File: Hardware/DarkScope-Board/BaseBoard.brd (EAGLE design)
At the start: 101.9 x 80 mm, 85 parts, among them IC1 7805DT, IC2 REG1117, IC3 7905, J1 DCJ0202, Q1 8MHz, T2 9014, U1 STM32F103CBT6, X1 TSW-102-07-G-S, X2 TSW-102-07-G-S, X3 MINI-USB-32005-301, X4 2540-5

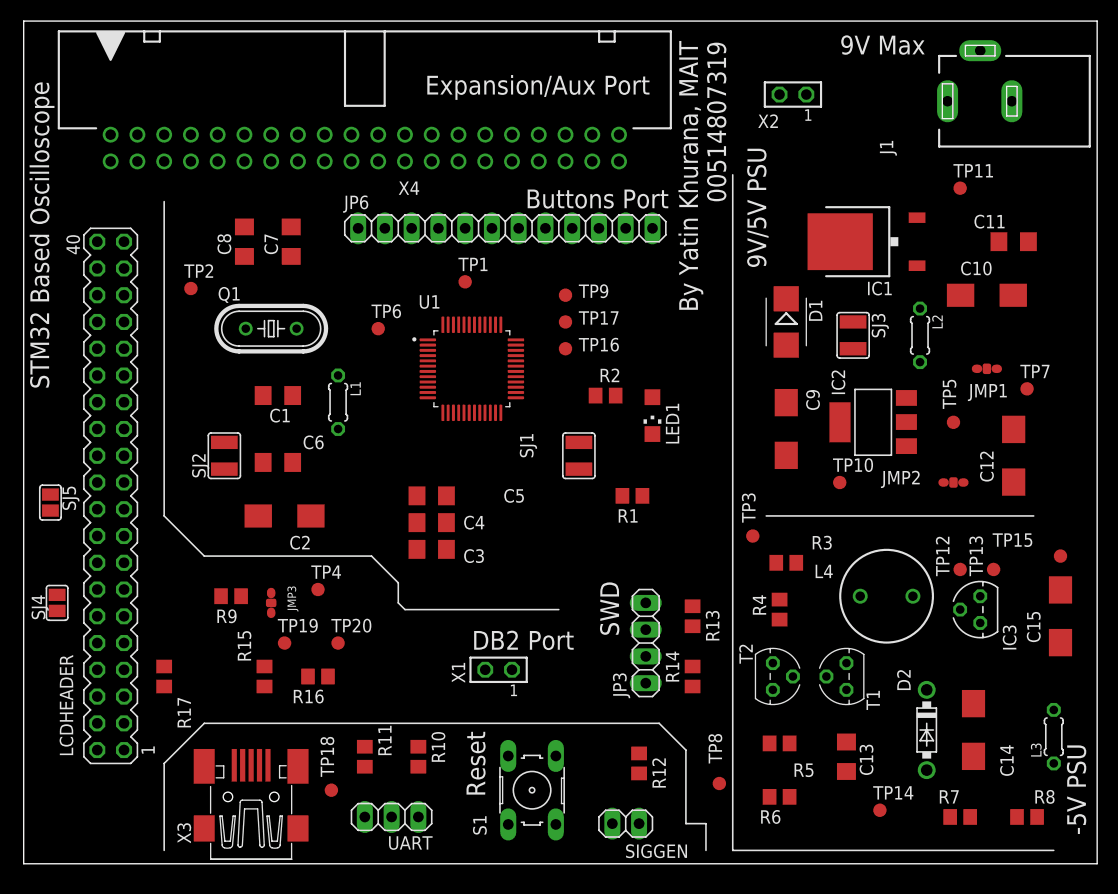
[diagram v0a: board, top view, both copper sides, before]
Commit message: CP BB PCB Draft
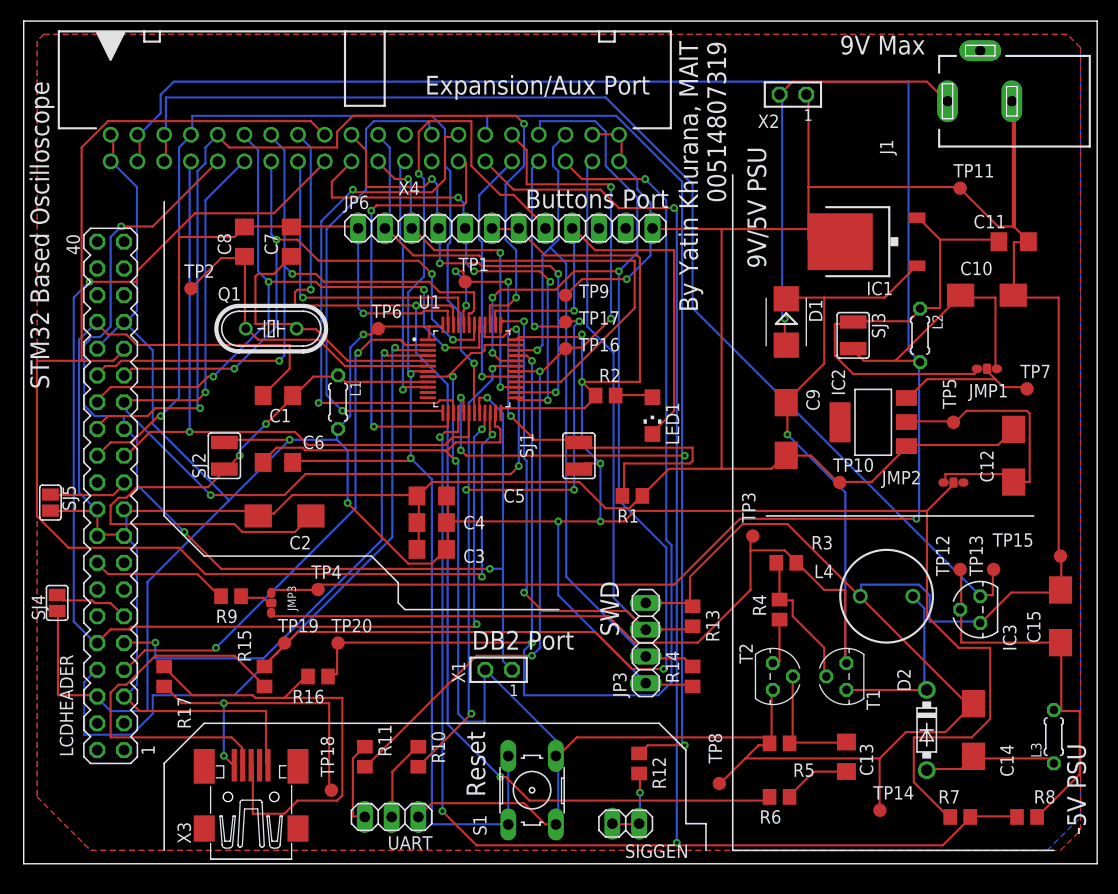
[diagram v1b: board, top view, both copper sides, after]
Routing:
- net GND: track 0.00 -> 634.1 mm, vias 0 -> 4
- net +3V3: track 0.00 -> 334.0 mm, vias 0 -> 8
- net +5V: track 0.00 -> 211.5 mm, vias 0 -> 1
- net V-MON: track 0.00 -> 176.8 mm, vias 0 -> 4
- net LCD_NRESET: track 0.00 -> 129.3 mm, vias 0 -> 2
- net USBDP: track 0.00 -> 127.8 mm, vias 0 -> 3
- net USBDM: track 0.00 -> 124.8 mm, vias 0 -> 4
- net +12V: track 0.00 -> 123.9 mm, vias 0 -> 1
- net LCD_NRD: track 0.00 -> 121.1 mm, vias 0 -> 3
- net -5V: track 0.00 -> 113.9 mm
- net NRST: track 0.00 -> 113.6 mm, vias 0 -> 3
- net TESTSIG: track 0.00 -> 109.7 mm, vias 0 -> 4
- net VGEN: track 0.00 -> 109.5 mm, vias 0 -> 3
- net DB2: track 0.00 -> 109.1 mm, vias 0 -> 4
- net SWCLK: track 0.00 -> 93.0 mm, vias 0 -> 2
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- added copper zone on layer 1, net GND
- added copper zone on layer 16, net GND
